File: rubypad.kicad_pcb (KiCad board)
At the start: 2 copper layers, 65 x 72 mm, 34 parts, among them J1 HRO-TYPE-C, SW1 SW_Push, SW2 RotaryEncoder_Switch, U1 ATmega32U4-A, Y1 16MHz

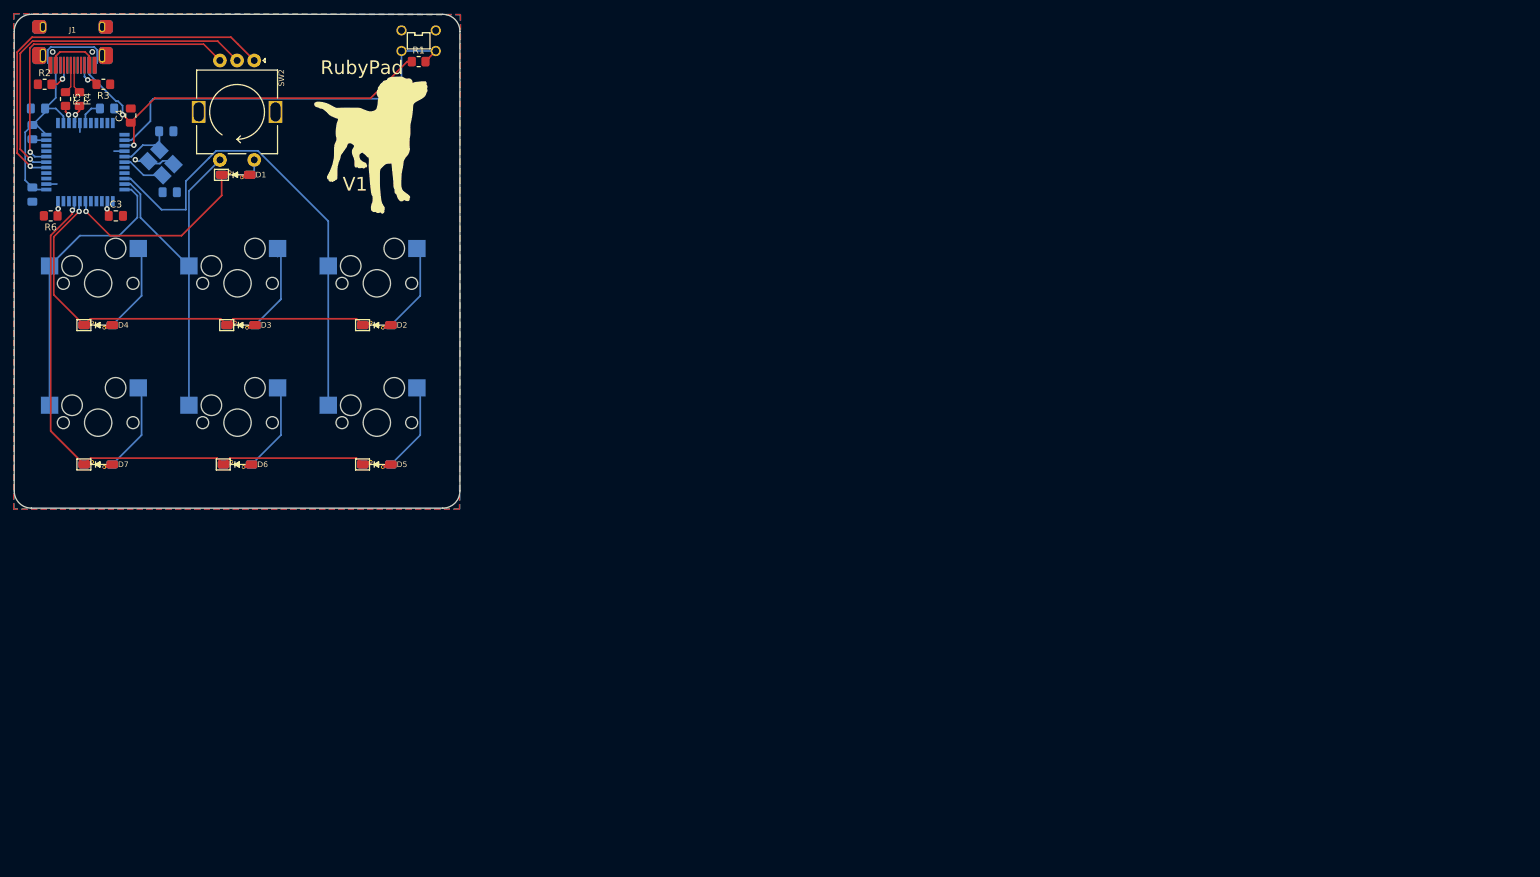
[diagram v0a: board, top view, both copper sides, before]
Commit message: udpate
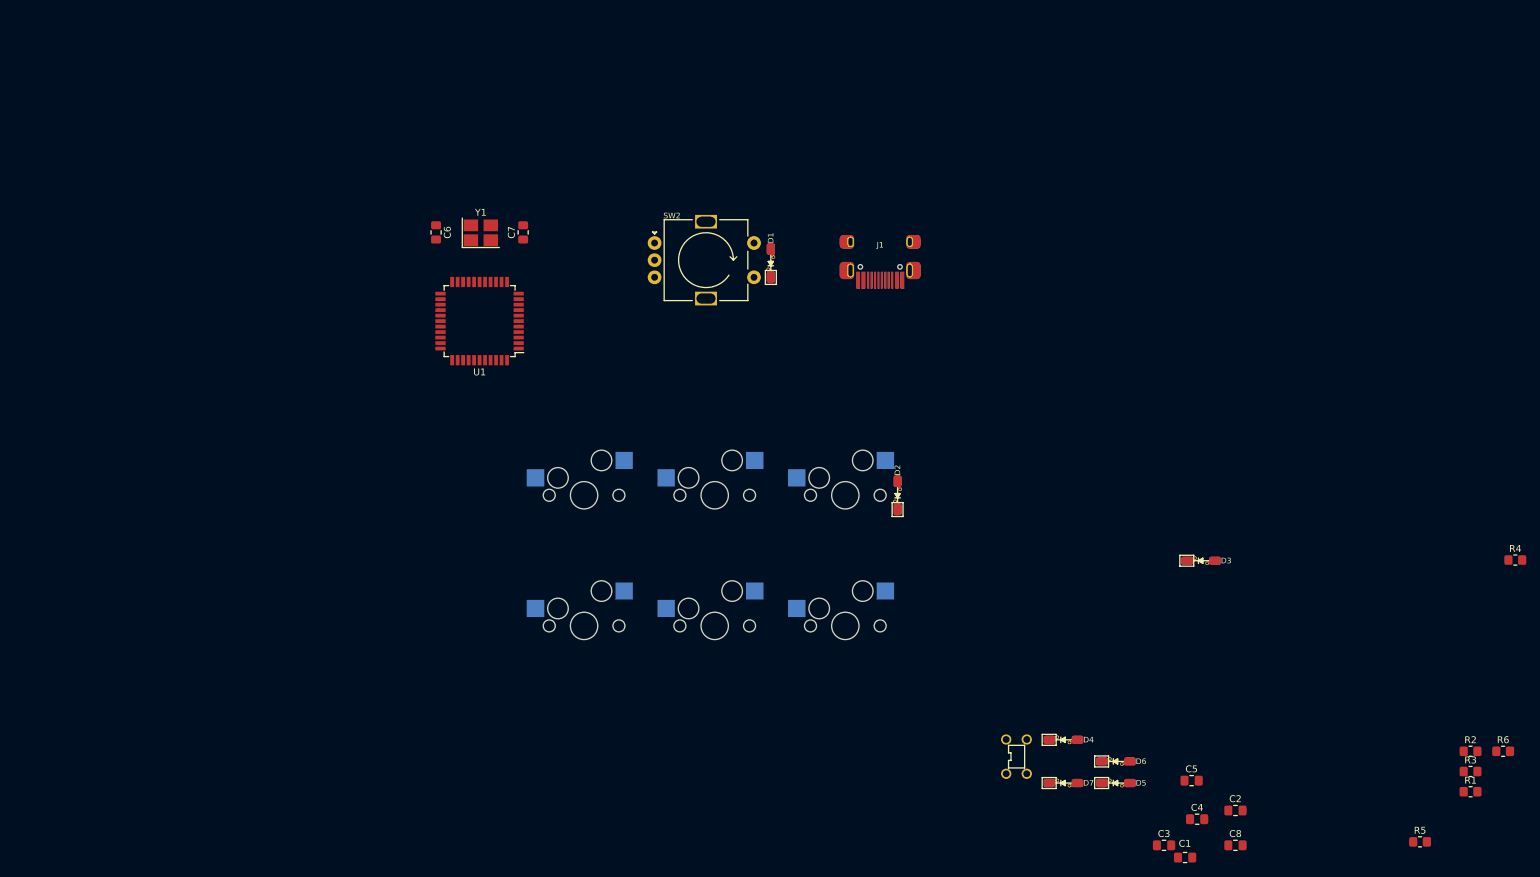
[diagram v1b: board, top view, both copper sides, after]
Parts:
- removed G*** (x2): LOGO, rubypad-footprints:logo
- C1, C2, C5, C6, C7, C8, U1: moved to F.Cu
- J1: moved to B.Cu
- Y1: footprint Crystal:Crystal_SMD_3225-4Pin_3.2x2.5mm_HandSoldering -> Crystal:Crystal_SMD_SeikoEpson_TSX3225-4Pin_3.2x2.5mm_HandSoldering; moved to F.Cu
- moved R2 229.6 mm to (247.4, 142.7)
- moved R6 225.8 mm to (252.1, 142.7), turned to 0 degrees
- moved R5 225.3 mm to (240.0, 156.0), turned to 0 degrees
- moved R3 223.2 mm to (247.4, 145.7), turned to 0 degrees
- moved R4 219.9 mm to (253.9, 114.9), turned to 0 degrees
- moved C2 202.4 mm to (213.1, 151.4), turned to 0 degrees
- moved C8 196.5 mm to (213.1, 156.5)
- moved C1 193.9 mm to (205.8, 158.2), turned to 0 degrees
- moved C5 193.7 mm to (206.7, 147.0), turned to 0 degrees
- moved R1 186.7 mm to (247.4, 148.6)
- moved C4 186.3 mm to (207.5, 152.7), turned to 0 degrees
- moved C3 178.3 mm to (202.7, 156.5)
- moved D4 153.2 mm to (188.0, 141.1)
- moved D7 148.2 mm to (188.0, 147.4)
- moved D3 144.2 mm to (208.1, 115.0)
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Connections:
- U1 pad 20: col0 -> unconnected-(U1-Pad20)
- U1 pad 21: col1 -> unconnected-(U1-Pad21)
- U1 pad 22: col2 -> unconnected-(U1-Pad22)
- U1 pad 28: row0 -> unconnected-(U1-Pad28)
- U1 pad 29: row1 -> unconnected-(U1-Pad29)
- U1 pad 30: row2 -> unconnected-(U1-Pad30)
- U1 pad 38: encA -> unconnected-(U1-Pad38)
- U1 pad 39: encC -> unconnected-(U1-Pad39)
- U1 pad 40: encB -> unconnected-(U1-Pad40)
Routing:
- net VCC: track 100.0 -> 0.00 mm, vias 3 -> 0
- net row2: track 84.0 -> 0.00 mm, vias 1 -> 0
- net col0: track 68.7 -> 0.00 mm
- net row1: track 63.7 -> 0.00 mm, vias 1 -> 0
- net Net-(R1-Pad2): track 57.0 -> 0.00 mm
- net encA: track 56.7 -> 0.00 mm, vias 1 -> 0
- net col1: track 54.0 -> 0.00 mm
- net encC: track 52.1 -> 0.00 mm, vias 1 -> 0
- net encB: track 46.8 -> 0.00 mm, vias 1 -> 0
- net col2: track 41.5 -> 0.00 mm
- net row0: track 28.2 -> 0.00 mm, vias 1 -> 0
- net GND: track 24.9 -> 0.00 mm, vias 1 -> 0
- net Net-(D3-Pad2): track 14.1 -> 0.00 mm
- net Net-(D6-Pad2): track 13.2 -> 0.00 mm
- net Net-(D7-Pad2): track 13.2 -> 0.00 mm
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- removed copper zone on B.Cu, net GND
- removed copper zone on F.Cu, net GND
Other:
- board outline removed
